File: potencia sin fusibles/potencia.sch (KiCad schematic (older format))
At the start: 17 parts

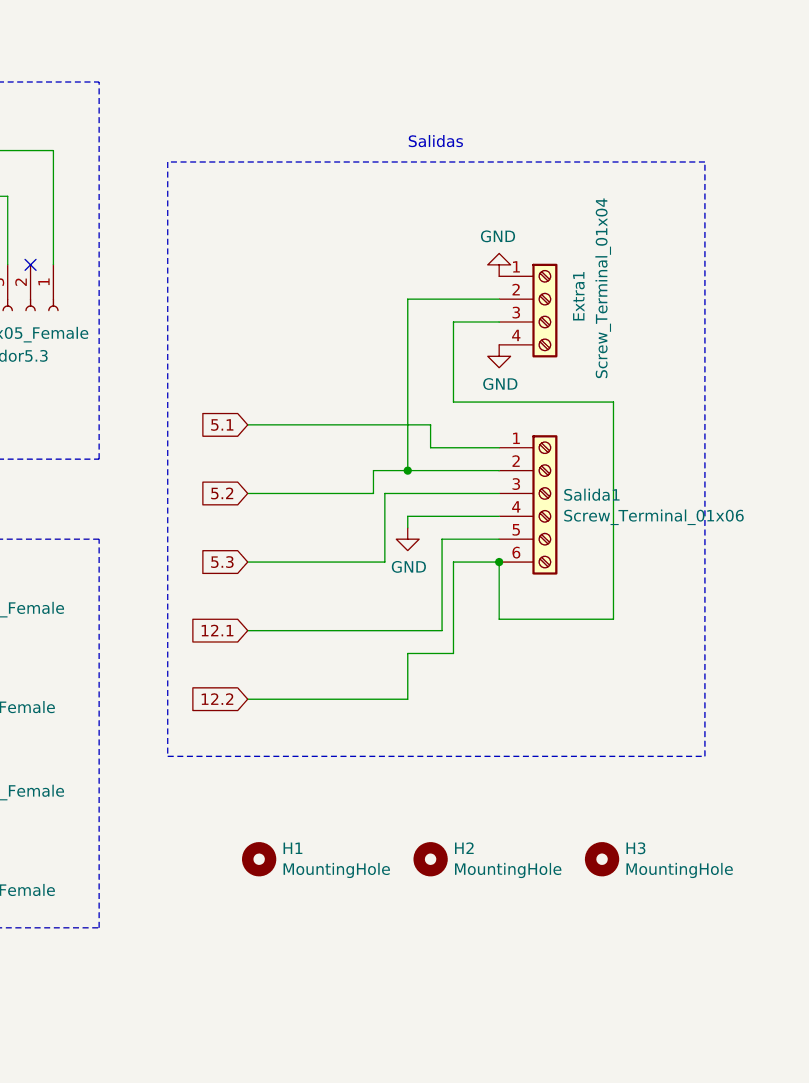
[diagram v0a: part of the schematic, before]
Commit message: version v2
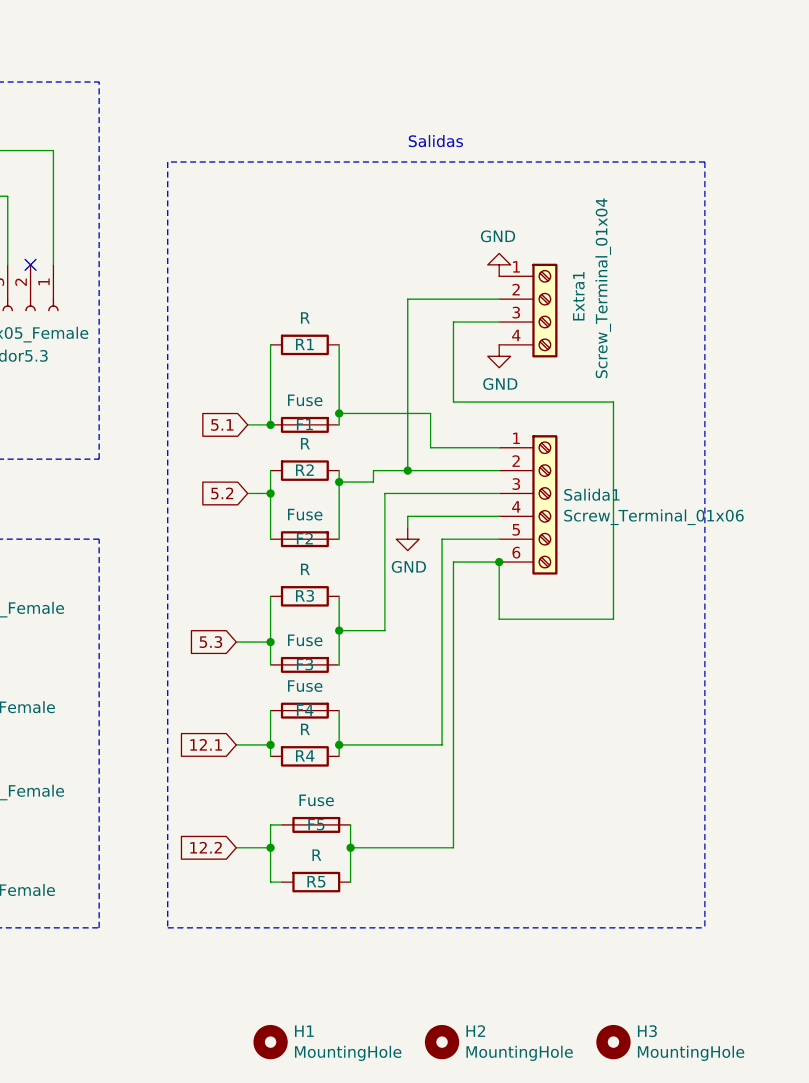
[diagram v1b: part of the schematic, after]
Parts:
- added F1, F2, F3, F4, F5: Fuse, symbol Device:Fuse
- added R1, R2, R3, R4, R5: R, Resistor_THT:R_Axial_DIN0204_L3.6mm_D1.6mm_P5.08mm_Horizontal, symbol Device:R
- Alimentación1, Extra1: footprint Connector_Phoenix_MC_HighVoltage:PhoenixContact_MCV_1,5_4-G-5.08_1x04_P5.08mm_Vertical -> Conector_Eurobot:Conector_4p_5.08
- Salida1: footprint Connector_Phoenix_MC_HighVoltage:PhoenixContact_MCV_1,5_6-G-5.08_1x06_P5.08mm_Vertical -> Conector_Eurobot:Conector_6p_5.08
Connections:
- net 12.1: now also F4.1, R4.2; no longer Salida1.5 (Pin_5)
- net 12.2: now also F5.1, R5.2; no longer Extra1.3 (Pin_3), Salida1.6 (Pin_6)
- net 5.1: now also F1.1, R1.2; no longer Salida1.1 (Pin_1)
- net 5.2: now also F2.1, R2.2; no longer Extra1.2 (Pin_2), Salida1.2 (Pin_2)
- net 5.3: now also F3.1, R3.2; no longer Salida1.3 (Pin_3)
- new net: Extra1.2 (Pin_2), F2.2, R2.1, Salida1.2 (Pin_2)
- new net: Extra1.3 (Pin_3), F5.2, R5.1, Salida1.6 (Pin_6)
- new net: F1.2, R1.1, Salida1.1 (Pin_1)
- new net: F3.2, R3.1, Salida1.3 (Pin_3)
- new net: F4.2, R4.1, Salida1.5 (Pin_5)
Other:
- moved on the sheet: H1, H2, H3
